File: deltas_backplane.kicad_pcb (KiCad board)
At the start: 2 copper layers, 143.5 x 119.2 mm, 16 parts, among them J1 SNP_female_straight, J2 SNP_female_straight, J3 SNP_female_straight, J4 SNP_female_straight, J5 SNP_male_angle, J6 zx_bus, J7 zx_bus, J8 Ext. Power (5V), J9 Conn_01x04

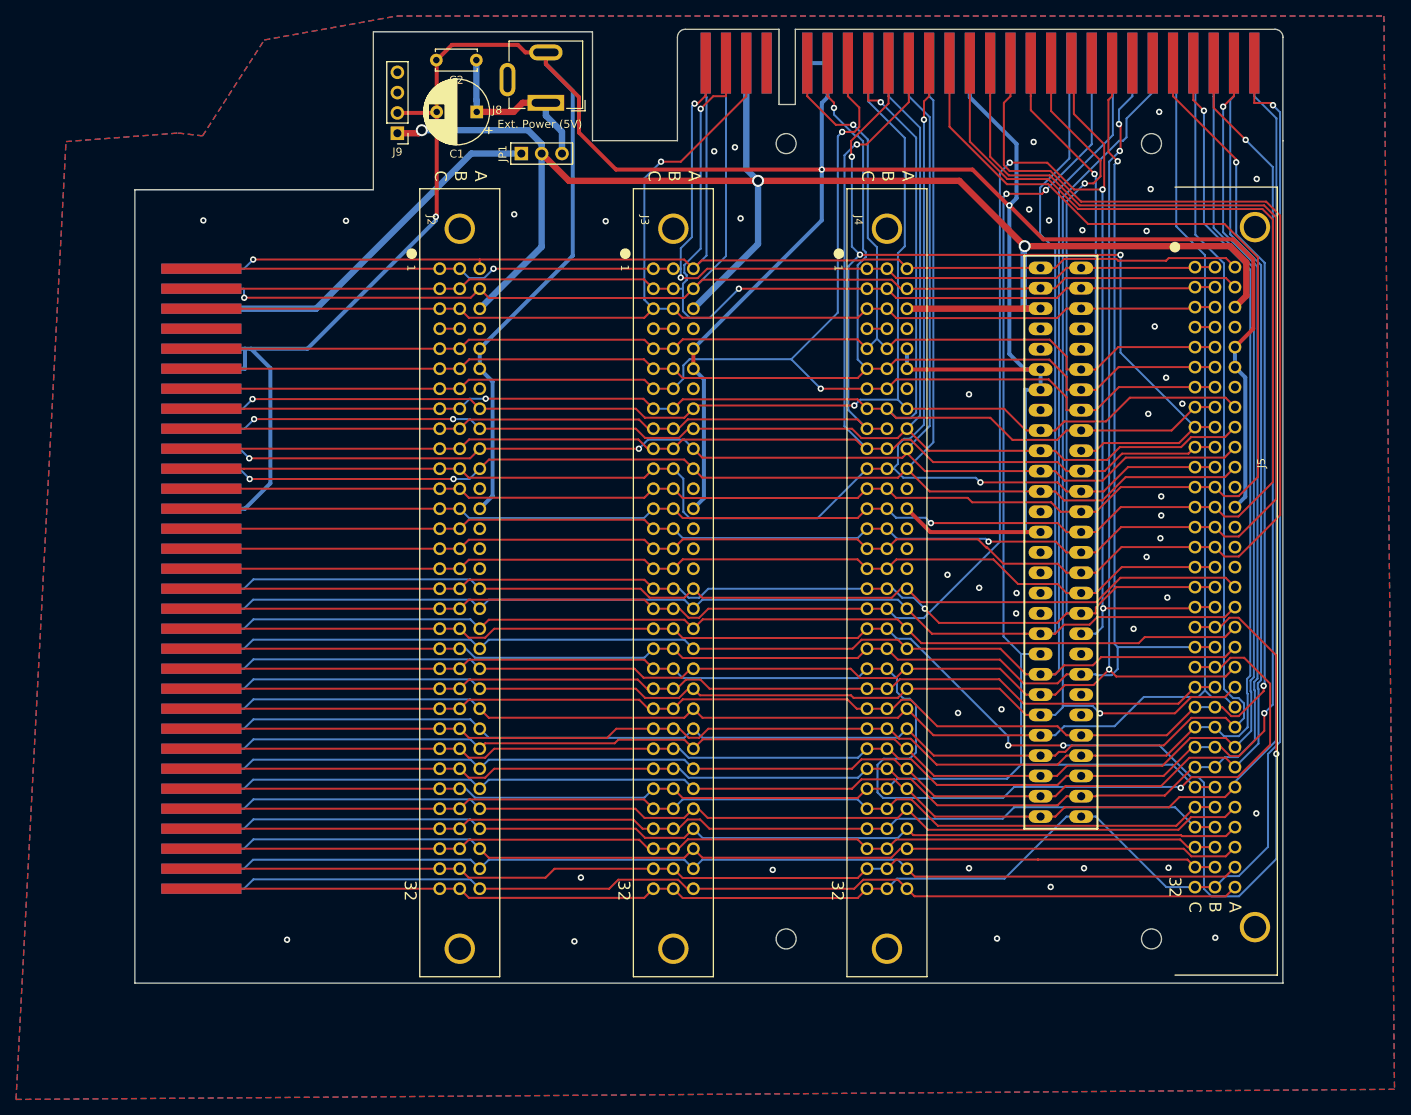
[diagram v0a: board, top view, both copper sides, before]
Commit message: Update deltas_backplane.kicad_pcb
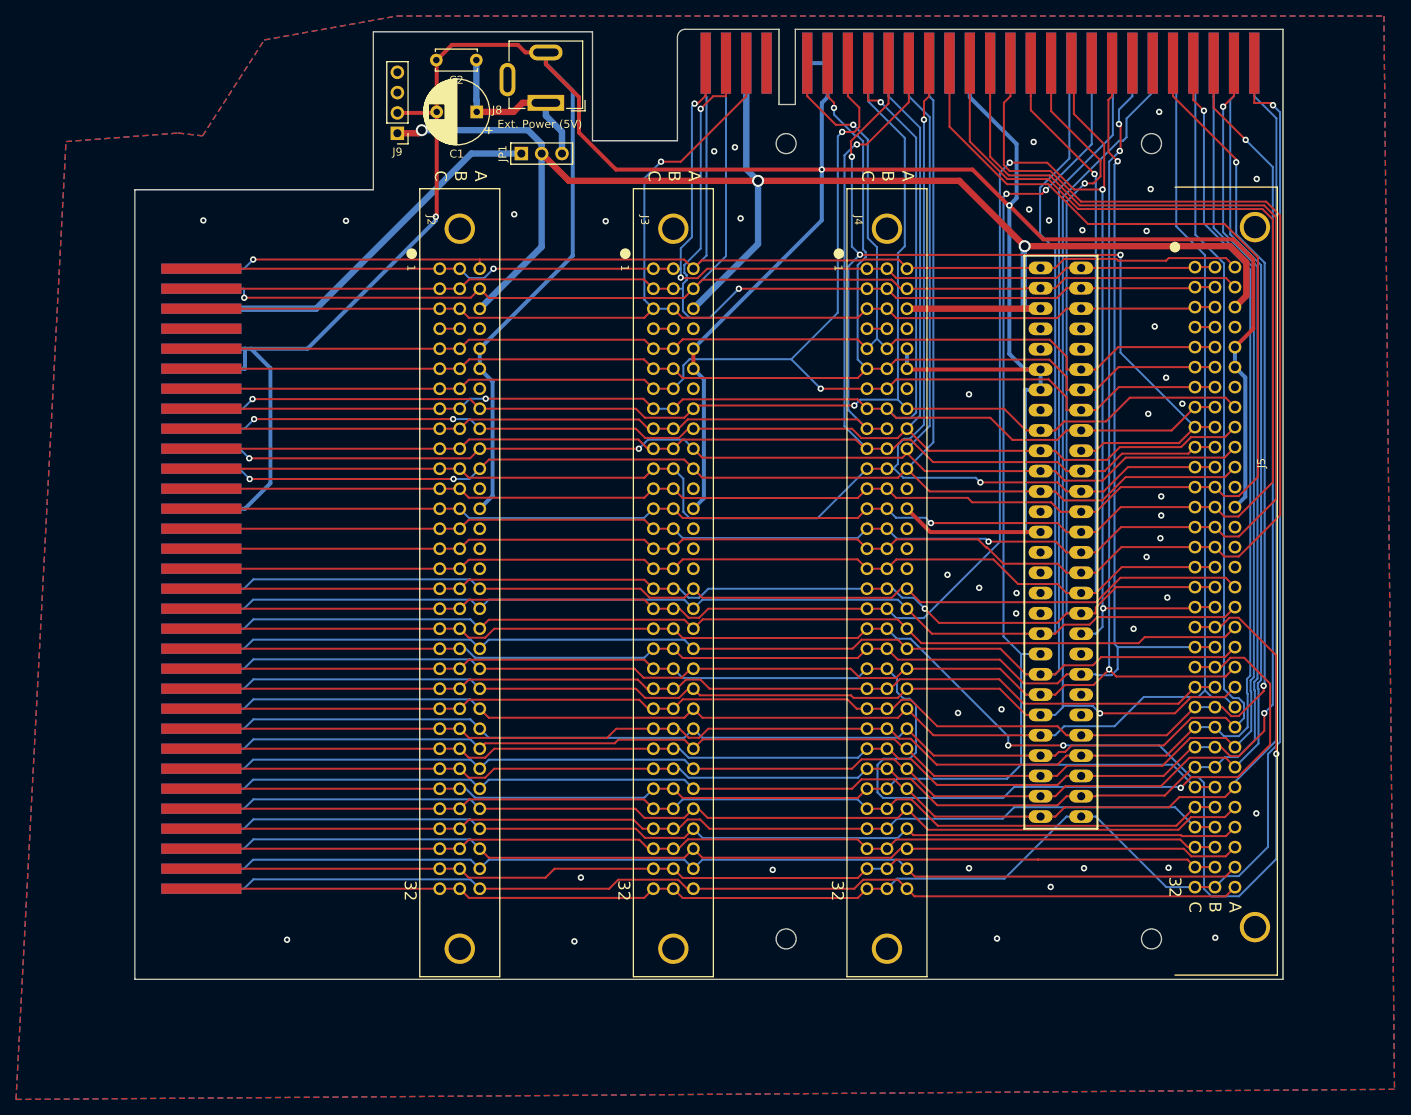
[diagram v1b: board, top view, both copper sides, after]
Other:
- board size 143.5 x 119.2 mm -> 143.5 x 118.8 mm
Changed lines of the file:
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@@
   (gr_line (start 167.74399 25.64352) (end 165.71199 25.64352)
     (stroke (width 0.1) (type solid)) (layer "Edge.Cuts"))
-  (gr_line (start 228.70399 135.47501) (end 85.19798 135.47501)
+  (gr_line (start 228.70399 135) (end 85.19798 135)
     (stroke (width 0.1) (type default)) (layer "Edge.Cuts"))
   (gr_arc (start 153.01199 17.24552) (mid 153.30488 16.538407) (end 154.01199 16.24552)
@@
   (gr_line (start 167.74399 16.24552) (end 167.74399 25.64352)
     (stroke (width 0.1) (type solid)) (layer "Edge.Cuts"))
-  (gr_line (start 227.70399 16.24552) (end 167.74399 16.24552)
+  (gr_line (start 228.70399 16.24552) (end 167.74399 16.24552)
     (stroke (width 0.1) (type solid)) (layer "Edge.Cuts"))
   (gr_line (start 115 36.30402) (end 115 16.56352)
     (stroke (width 0.1) (type default)) (layer "Edge.Cuts"))
-  (gr_line (start 228.70399 30.17701) (end 228.70399 135.47501)
+  (gr_line (start 228.70399 16.24552) (end 228.70399 135)
     (stroke (width 0.1) (type default)) (layer "Edge.Cuts"))
-  (gr_line (start 85.19798 36.30402) (end 85.19798 135.47501)
-    (stroke (width 0.1) (type solid)) (layer "Edge.Cuts"))
-  (gr_line (start 228.70399 30.17701) (end 228.70399 17.24552)
+  (gr_line (start 85.19798 36.30402) (end 85.19798 135)
     (stroke (width 0.1) (type solid)) (layer "Edge.Cuts"))
   (gr_line (start 85.19798 36.30402) (end 115 36.30402)
     (stroke (width 0.1) (type default)) (layer "Edge.Cuts"))
-  (gr_arc (start 227.70399 16.24552) (mid 228.411093 16.538414) (end 228.70399 17.24552)
-    (stroke (width 0.1) (type default)) (layer "Edge.Cuts"))
   (gr_line (start 142.39299 16.56352) (end 142.39299 30.17701)
